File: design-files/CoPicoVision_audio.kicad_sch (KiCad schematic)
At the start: 9 parts, among them J501 AudioJack3, Q501 KSD1616A, U501 SN76489AN

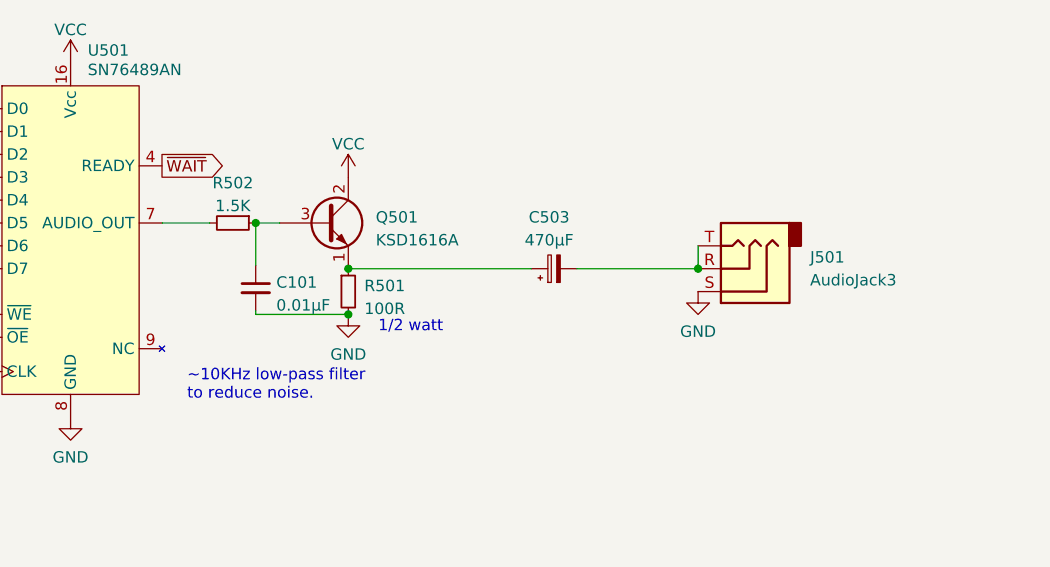
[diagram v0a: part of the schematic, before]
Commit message: Project update, and use a TL071 opamp for the audio output buffer.
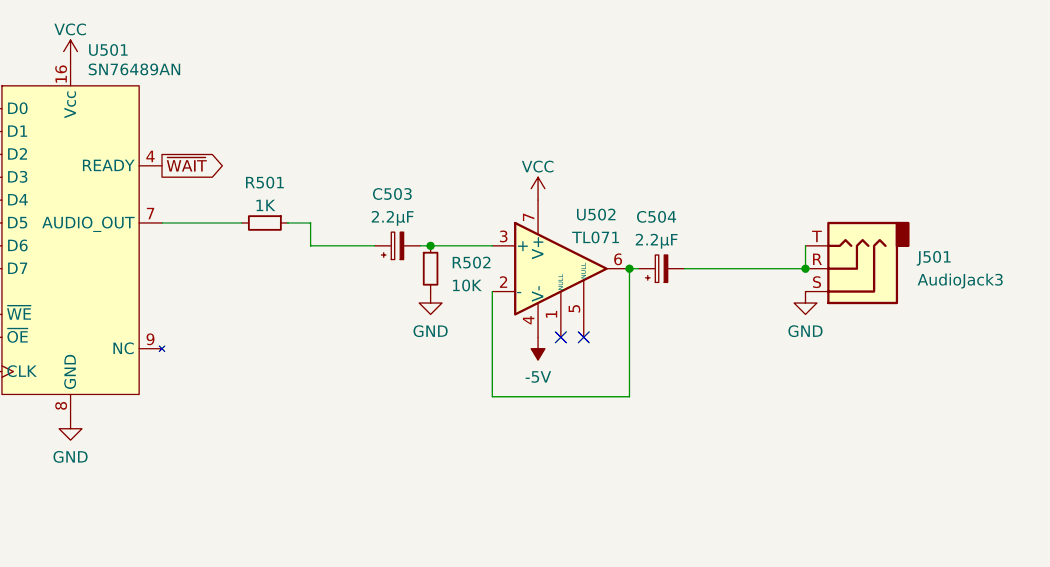
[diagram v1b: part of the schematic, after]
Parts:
- removed C101: 0.01µF, Capacitor_THT:C_Disc_D3.8mm_W2.6mm_P2.50mm, symbol Device:C_Small
- removed Q501: KSD1616A, Package_TO_SOT_THT:TO-92L_Inline_Wide, symbol Device:Q_NPN_ECB
- removed R501: 100R, Resistor_THT:R_Axial_DIN0207_L6.3mm_D2.5mm_P2.54mm_Vertical, symbol Device:R_Small
- added C504: 2.2µF, Capacitor_THT:CP_Radial_D6.3mm_P2.50mm, symbol Device:C_Polarized_Small
- added R502: 10K, Resistor_SMD:R_0805_2012Metric_Pad1.20x1.40mm_HandSolder, symbol Device:R_Small
- added U502: TL071, Package_DIP:DIP-8_W7.62mm_Socket, symbol Amplifier_Operational:TL071
- C503: value 470µF -> 2.2µF
- R501: renamed from R502; value 1.5K -> 1K; footprint Resistor_THT:R_Axial_DIN0207_L6.3mm_D2.5mm_P2.54mm_Vertical -> Resistor_SMD:R_0805_2012Metric_Pad1.20x1.40mm_HandSolder
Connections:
- net GND: now also R502.2
- net VCC: now also U502.7 (V+)
- net at C503.1: now also R501.1
- net at J501.R, J501.T: now also C504.2; no longer C503.2
- new net: C503.2, R502.1, U502.3 (+)
- new net: C504.1, U502.2 (-), U502.6
- new net -5V: U502.4 (V-)
- no-connect marks 0 -> 2
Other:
- note removed: "1/2 watt"
- note removed: "~10KHz low-pass filter to reduce noise."
- moved on the sheet: C503, J501, R501

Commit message: All the bypass caps are now 0805s.
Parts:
- C201: footprint Capacitor_THT:C_Disc_D3.8mm_W2.6mm_P2.50mm -> Capacitor_SMD:C_0805_2012Metric_Pad1.18x1.45mm_HandSolder
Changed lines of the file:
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@@
       (effects (font (size 1.27 1.27)) (justify left))
     )
-    (property "Footprint" "Capacitor_THT:C_Disc_D3.8mm_W2.6mm_P2.50mm" (at 84.836 133.604 0)
+    (property "Footprint" "Capacitor_SMD:C_0805_2012Metric_Pad1.18x1.45mm_HandSolder" (at 84.836 133.604 0)
       (effects (font (size 1.27 1.27)) hide)
     )

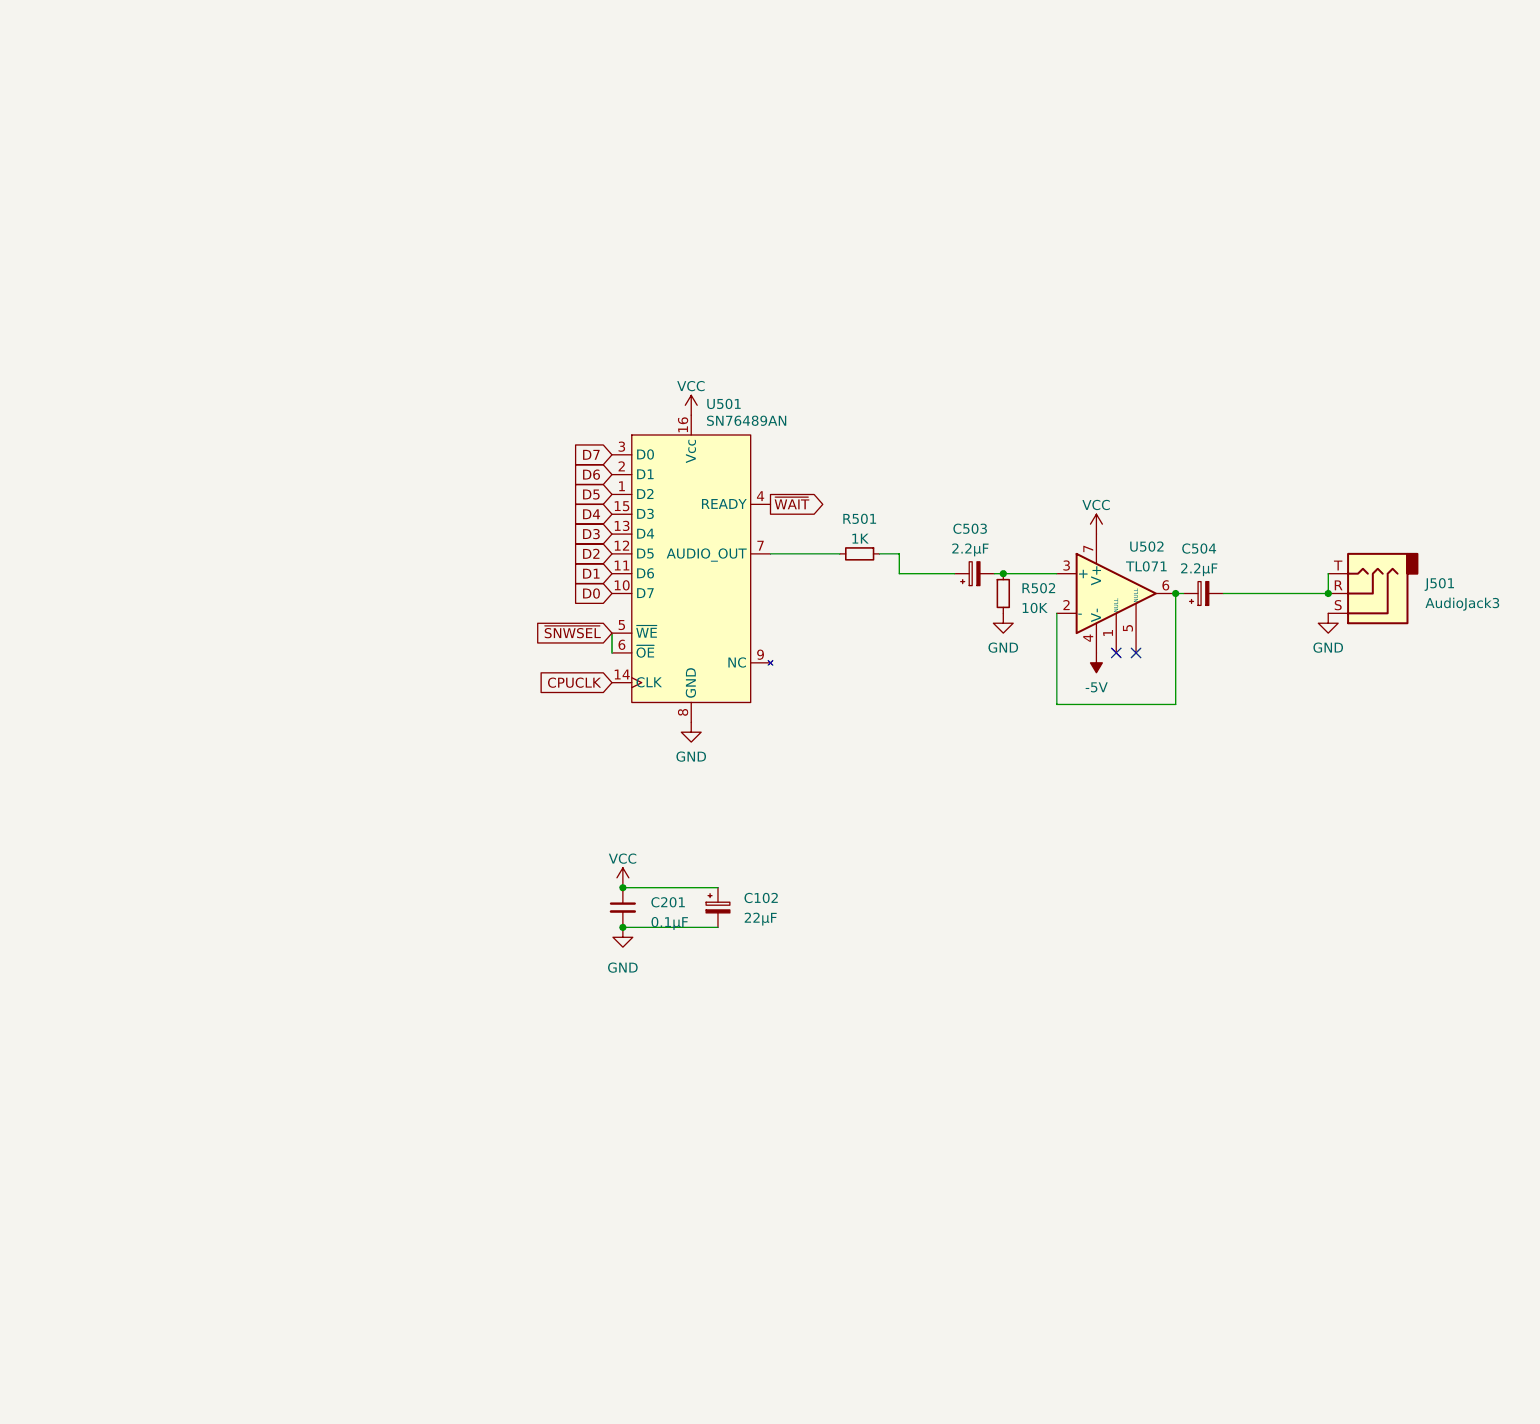
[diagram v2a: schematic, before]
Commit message: Put the AY-3-8910 on the schematic.  Need to make some more room on the board.
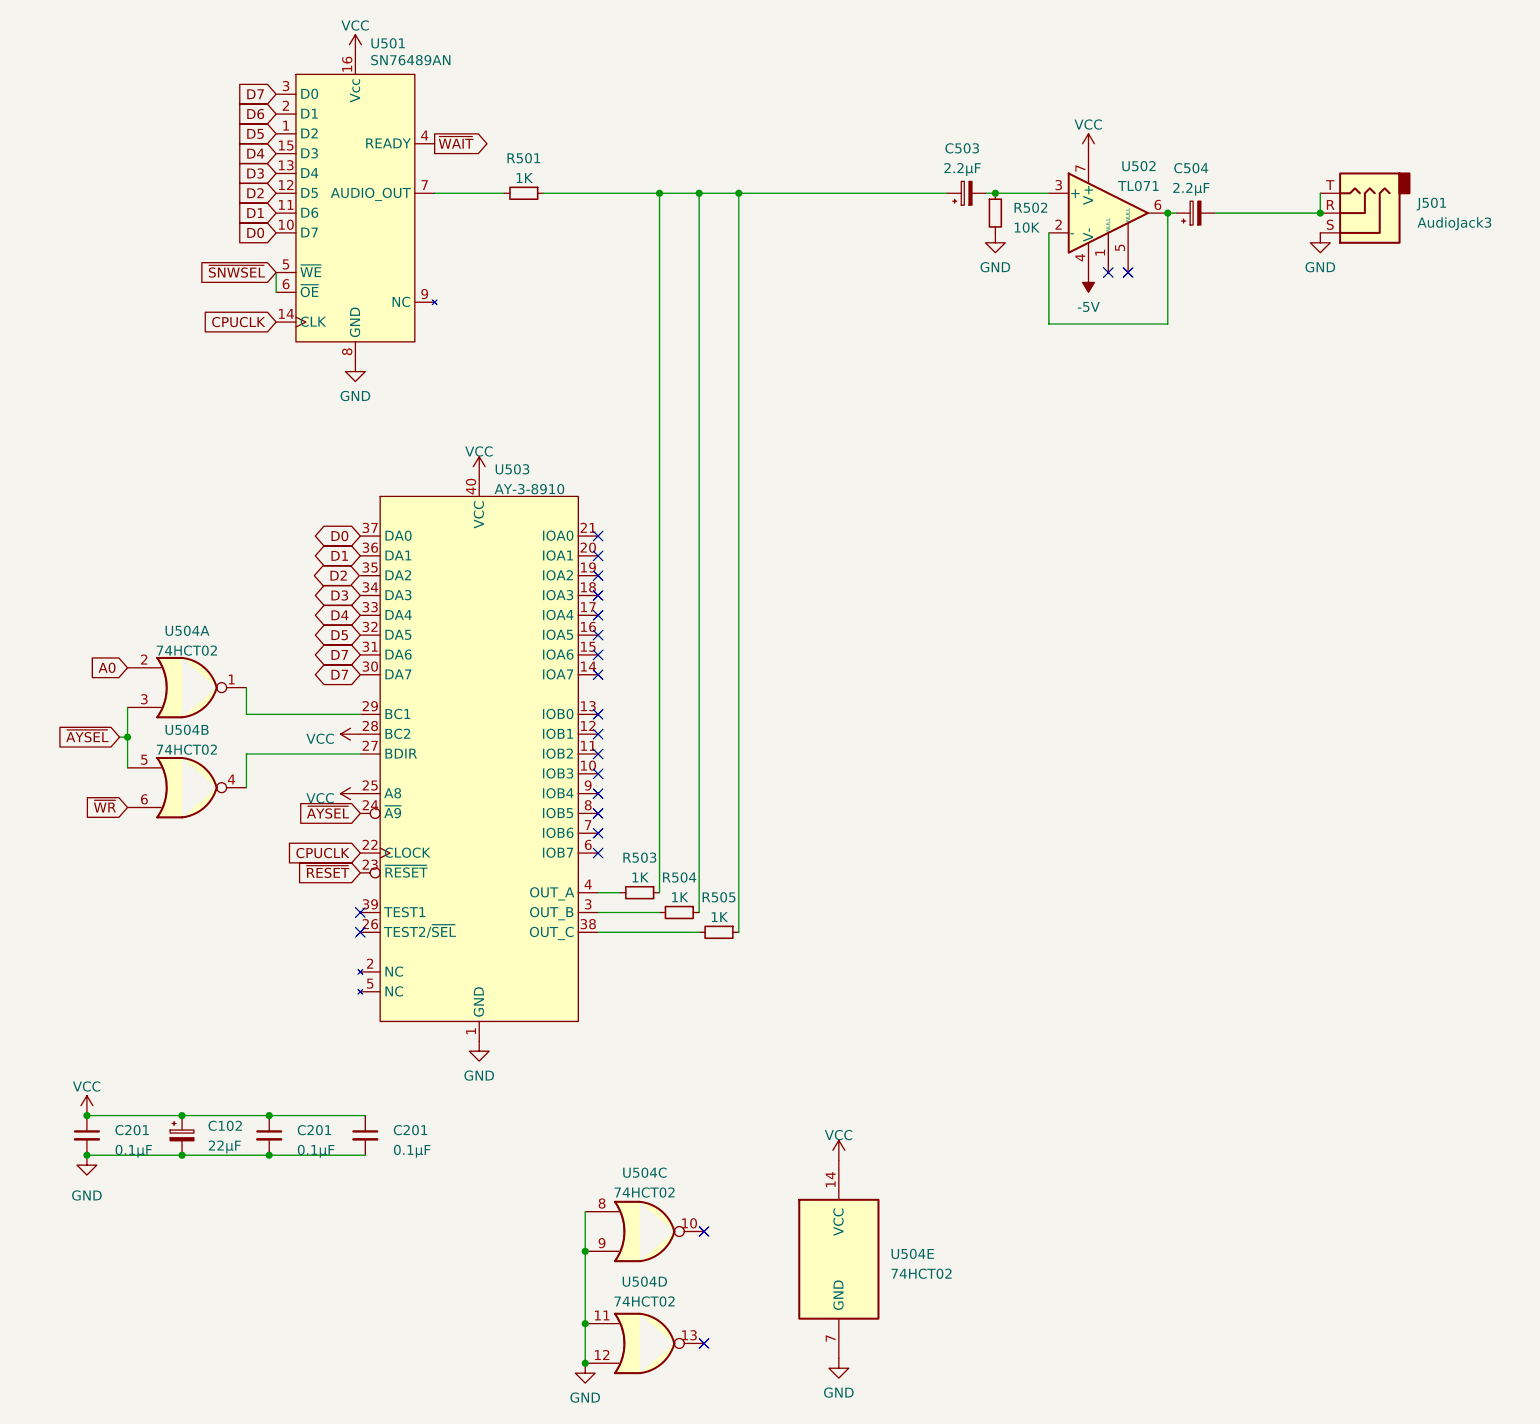
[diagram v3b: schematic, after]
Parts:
- added C201 (x2): 0.1µF, Capacitor_SMD:C_0805_2012Metric_Pad1.18x1.45mm_HandSolder, symbol Device:C_Small
- added R503, R504, R505: 1K, Resistor_SMD:R_0805_2012Metric_Pad1.20x1.40mm_HandSolder, symbol Device:R_Small
- added U503: AY-3-8910, Package_DIP:DIP-40_W15.24mm, symbol jrt-ICs:AY-3-8910
- added U504: 74HCT02, Package_SO:SOIC-14_3.9x8.7mm_P1.27mm, symbol 74xx:74HCT02
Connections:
- net CPUCLK: now also U503.22 (CLOCK)
- net D0: now also U503.37 (DA0)
- net D1: now also U503.36 (DA1)
- net D3: now also U503.34 (DA3)
- net D4: now also U503.33 (DA4)
- net D5: now also U503.32 (DA5)
- net D7: now also U503.30 (DA7), U503.31 (DA6)
- net GND: now also C201.2, C201.2, U503.1 (GND), U504.11, U504.12, U504.7 (GND), U504.8, U504.9
- net VCC: now also C201.1, C201.1, U503.25 (A8), U503.28 (BC2), U503.40 (VCC), U504.14 (VCC)
- net at C503.1, R501.1: now also R503.1, R504.1, R505.1
- new net: U503.29 (BC1), U504.1
- new net: R505.2, U503.38 (OUT_C)
- new net: U503.27 (BDIR), U504.4
- new net: R503.2, U503.4 (OUT_A)
- new net: R504.2, U503.3 (OUT_B)
- new net A0: U504.2
- new net ~{AYSEL}: U503.24 (~{A9}), U504.3, U504.5
- new net ~{RESET}: U503.23 (~{RESET})
- new net ~{WR}: U504.6
- no-connect marks 2 -> 22
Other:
- moved on the sheet: C102, C201, C503, C504, J501, R501, R502, U501, U502
